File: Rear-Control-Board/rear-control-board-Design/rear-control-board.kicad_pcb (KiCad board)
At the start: 2 copper layers, 139.1 x 102.8 mm, 55 parts, among them J1 Conn_01x23, J2 Conn_01x23, J3 Conn_01x08, J4 JST-B2B-VERT-2PIN, J5 JST-B2B-VERT-2PIN, J6 Conn_01x02, J7 Micro_SD_Card, K1 T9VV1K15-12S, K2 G5V-2, K3 G5V-2, Q2 PSMN5R2-60YL, Q3 PSMN5R2-60YL, Q4 PSMN5R2-60YL, U1 Dev_Board_C, U2 TS2940CP33 ROG, U4 MAX33054EASA+T

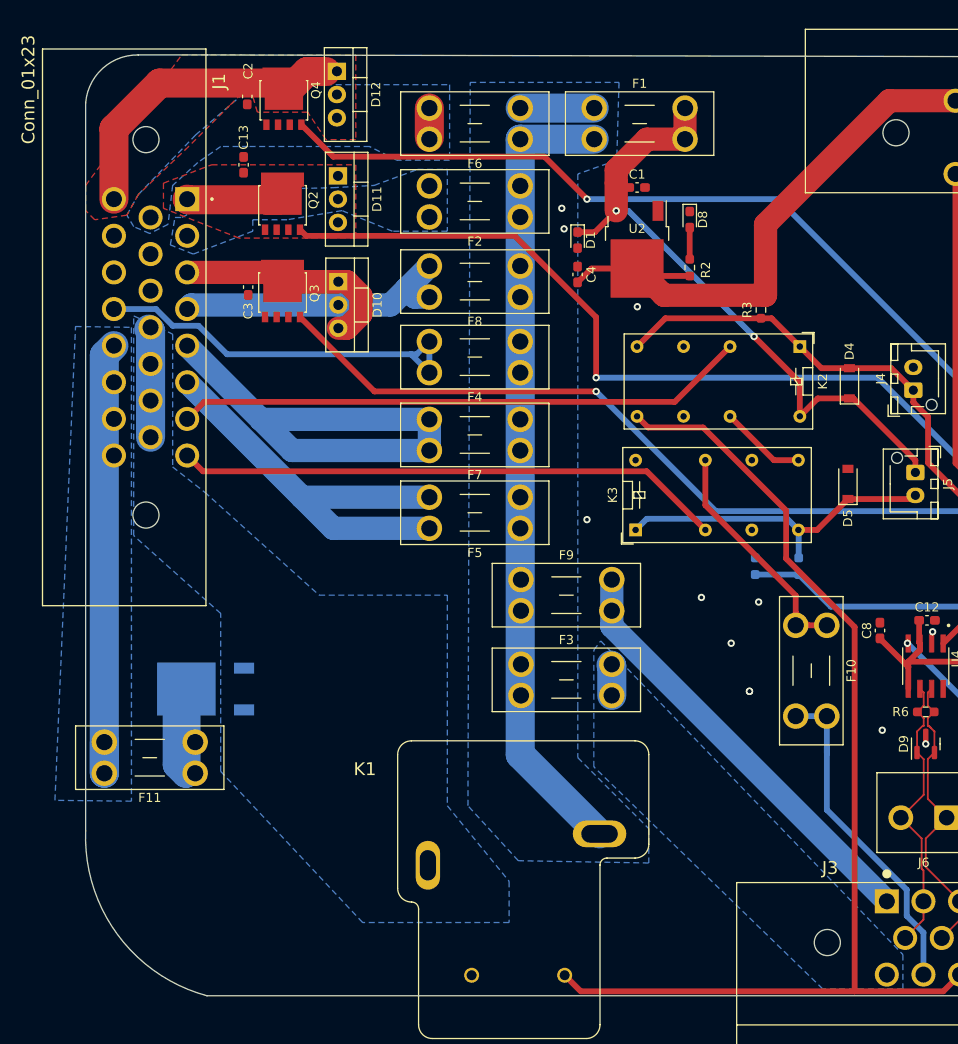
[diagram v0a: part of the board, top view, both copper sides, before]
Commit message: oops forgot to push for awile
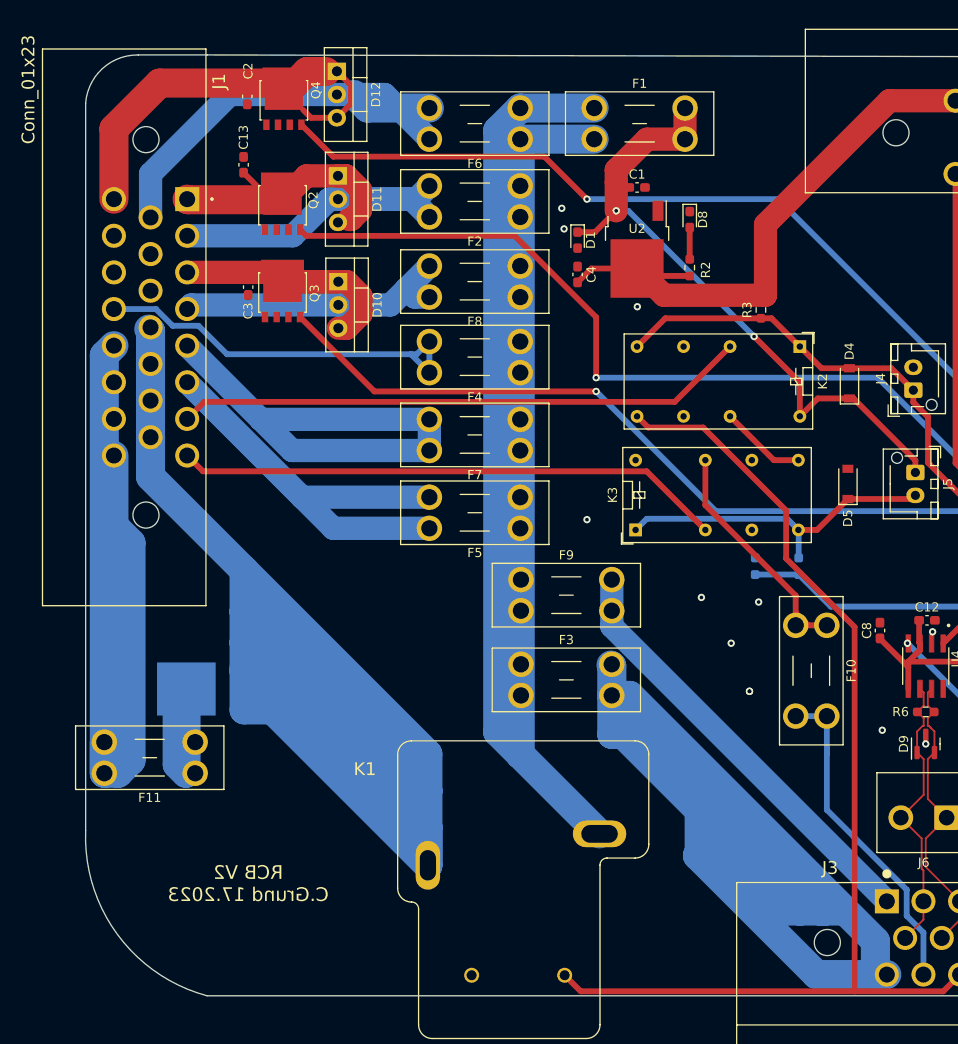
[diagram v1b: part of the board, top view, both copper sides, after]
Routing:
- net /BATT_12V: track 11.9 -> 184.1 mm
- net /RINE_12: track 3.35 -> 162.1 mm
- net +12V: track 95.6 -> 168.3 mm
- net /PUMP_12V: track 3.20 -> 49.6 mm
- net /FAN_12V: track 0.00 -> 40.4 mm
- net /DCDC_IN: track 50.5 -> 88.1 mm
- net /FAN_RTRN_12V: track 12.4 -> 30.4 mm
- net /PUMP_RTRN_12V: track 34.5 -> 44.9 mm
- removed copper zone on B.Cu, net +12V
- removed copper zone on B.Cu, net /BATT_12V
- removed copper zone on B.Cu, net /DCDC_IN
- removed copper zone on B.Cu, net /FAN_12V
- removed copper zone on F.Cu, net /FAN_RTRN_12V
- removed copper zone on B.Cu, net /PUMP_12V
- removed copper zone on F.Cu, net /PUMP_RTRN_12V
- removed copper zone on B.Cu, net /RINE_12
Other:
- board text added: "RCB V2 C.Grund 17.2023"
